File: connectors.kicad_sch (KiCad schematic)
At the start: 4 parts, among them J1 Conn_01x04_Pin, J2 Conn_01x04_Pin, J3 Conn_01x09_Pin, J4 Conn_02x03_Odd_Even

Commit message: Completed symbol footprint associations
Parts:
- J1, J2: footprint (none) -> Connector_PinHeader_2.54mm:PinHeader_1x04_P2.54mm_Vertical
- J3: footprint (none) -> Connector_PinHeader_2.54mm:PinHeader_1x09_P2.54mm_Vertical
- J4: footprint (none) -> Connector_PinHeader_2.54mm:PinHeader_2x03_P2.54mm_Vertical
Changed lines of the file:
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@@
 			)
 		)
-		(property "Footprint" ""
+		(property "Footprint" "Connector_PinHeader_2.54mm:PinHeader_2x03_P2.54mm_Vertical"
 			(at 158.75 106.68 0)
 			(effects
@@
 			)
 		)
-		(property "Footprint" ""
+		(property "Footprint" "Connector_PinHeader_2.54mm:PinHeader_1x04_P2.54mm_Vertical"
 			(at 125.73 67.31 0)
 			(effects
@@
 			)
 		)
-		(property "Footprint" ""
+		(property "Footprint" "Connector_PinHeader_2.54mm:PinHeader_1x04_P2.54mm_Vertical"
 			(at 156.21 67.31 0)
 			(effects
@@
 			)
 		)
-		(property "Footprint" ""
+		(property "Footprint" "Connector_PinHeader_2.54mm:PinHeader_1x09_P2.54mm_Vertical"
 			(at 128.27 113.03 0)
 			(effects

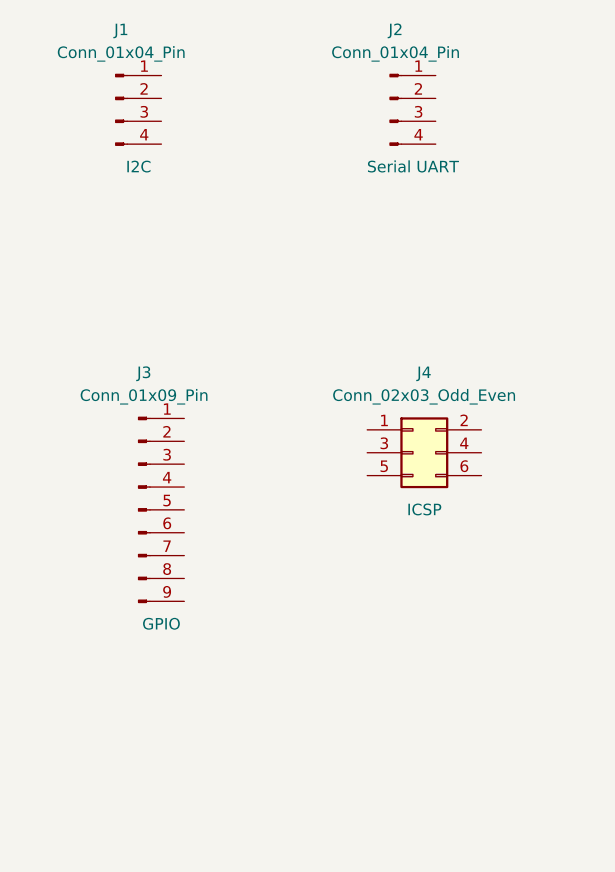
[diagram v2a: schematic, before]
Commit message: Complete wiring in the second sheet
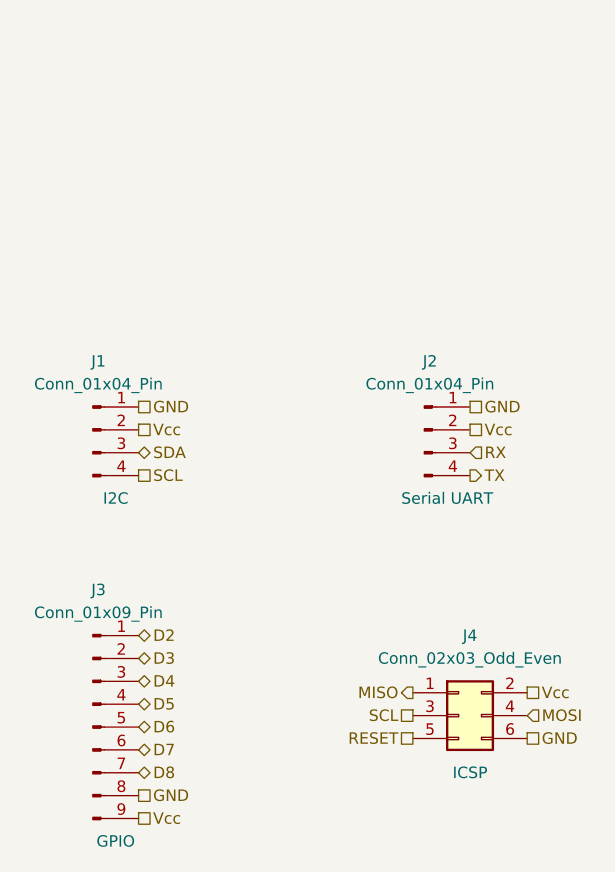
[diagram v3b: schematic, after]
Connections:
- net MISO: now reaches J4.1 (Pin_1)
- net Vcc: now reaches J4.2 (Pin_2)
- net Vcc: now also J1.2 (Pin_2), J2.2 (Pin_2), J3.9 (Pin_9)
- net SCL: now reaches J4.3 (Pin_3)
- net SCL: now also J1.4 (Pin_4)
- net MOSI: now reaches J4.4 (Pin_4)
- net RESET: now reaches J4.5 (Pin_5)
- net GND: now reaches J4.6 (Pin_6)
- net GND: now also J1.1 (Pin_1), J2.1 (Pin_1), J3.8 (Pin_8)
- net SDA: now reaches J1.3 (Pin_3)
- net RX: now reaches J2.3 (Pin_3)
- net TX: now reaches J2.4 (Pin_4)
- net D2: now reaches J3.1 (Pin_1)
- net D3: now reaches J3.2 (Pin_2)
- net D4: now reaches J3.3 (Pin_3)
- net D5: now reaches J3.4 (Pin_4)
- net D6: now reaches J3.5 (Pin_5)
- net D7: now reaches J3.6 (Pin_6)
- net D8: now reaches J3.7 (Pin_7)
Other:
- moved on the sheet: J1, J2, J3, J4
